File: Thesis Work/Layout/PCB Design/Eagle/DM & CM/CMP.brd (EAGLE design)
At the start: 46.3 x 19.4 mm, 7 parts, among them J1 SMA-J-P-H-ST-EM1, J2 SMA-J-P-H-ST-EM1

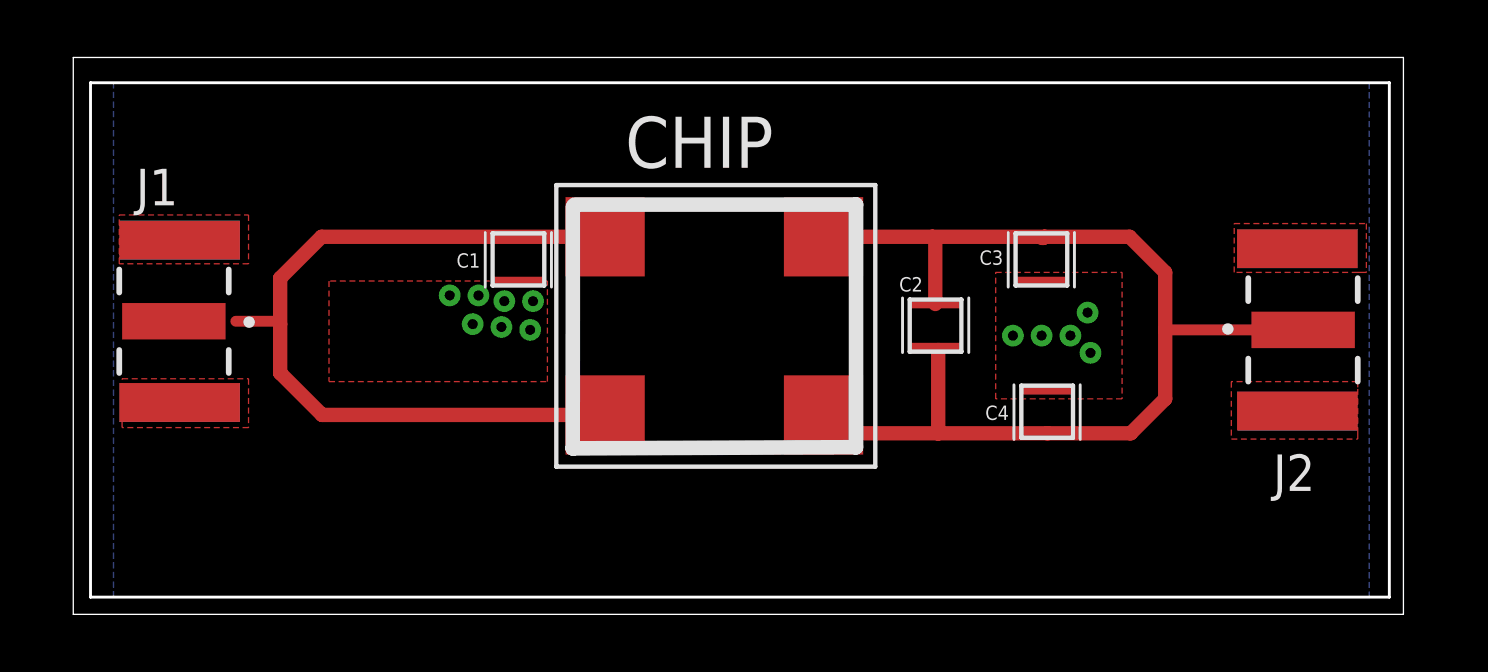
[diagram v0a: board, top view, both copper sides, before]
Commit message: c
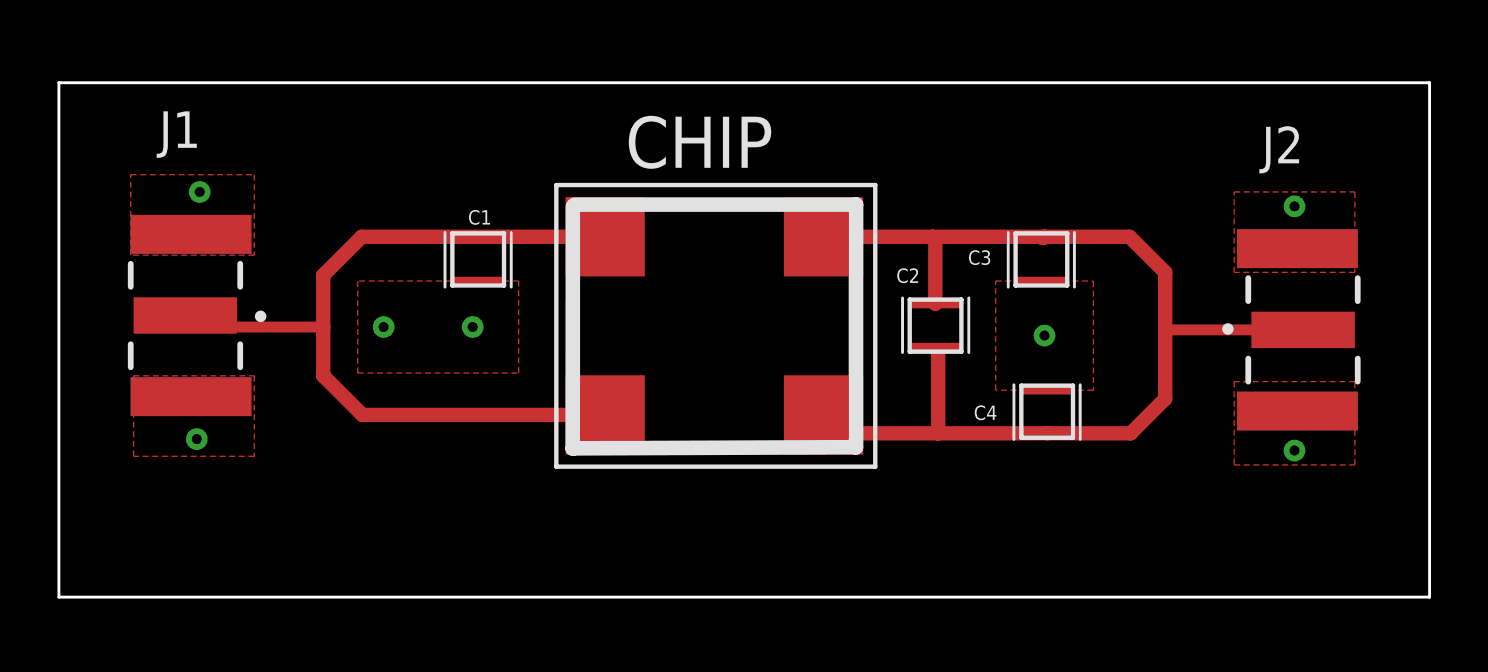
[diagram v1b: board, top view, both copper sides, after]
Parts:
- moved C1 1.40 mm to (31.6, 24.6)
- moved J1 0.45 mm to (21.4, 22.6)
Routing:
- net GND: vias 12 -> 7
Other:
- board size 46.3 x 19.4 mm -> 47.7 x 17.9 mm
